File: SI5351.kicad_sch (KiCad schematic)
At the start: 21 parts, among them U10 SI5351B-B-GM1, Y1 25MHz

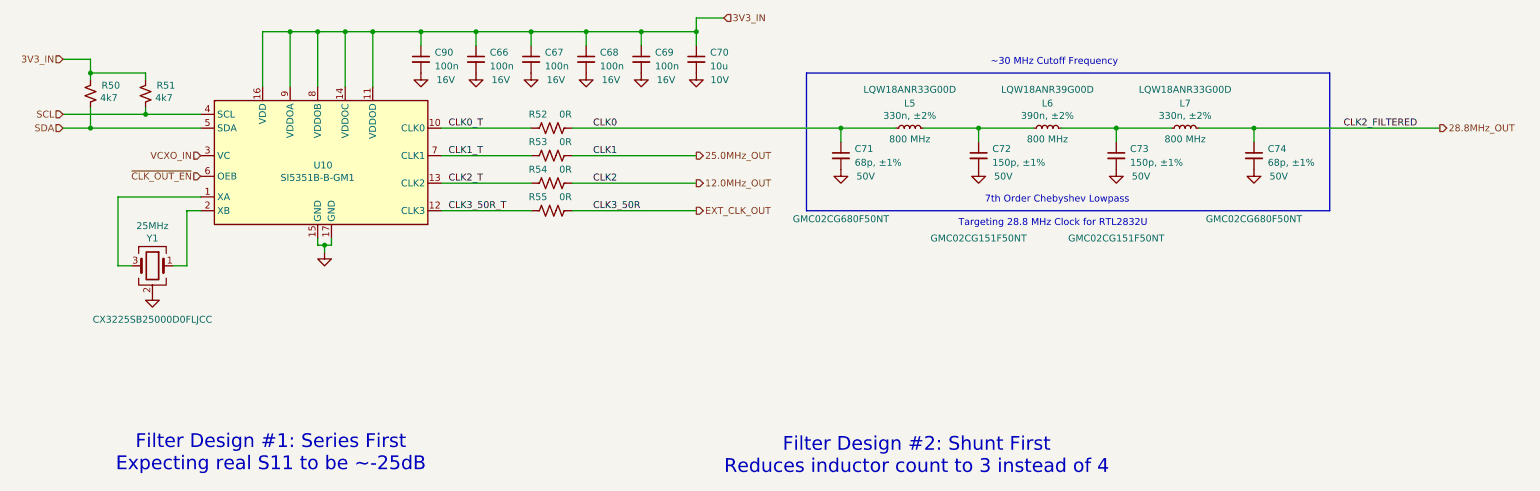
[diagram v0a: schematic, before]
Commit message: PCB and schematic progress
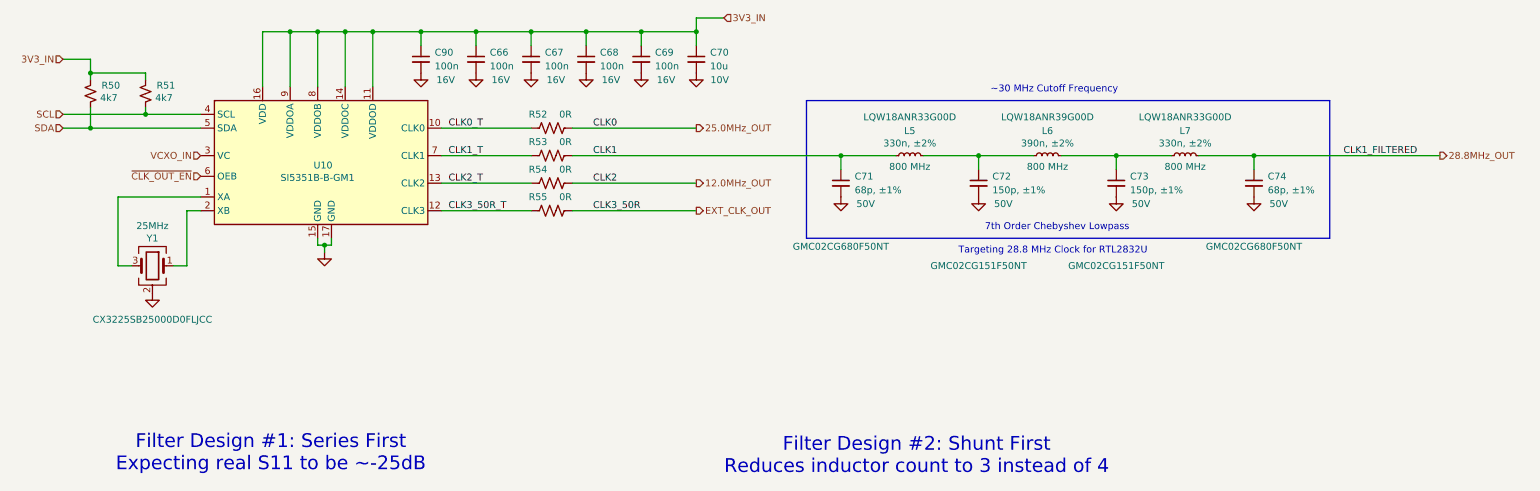
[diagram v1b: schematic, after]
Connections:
- net 25.0MHz_OUT: now also R52.2; no longer R53.2
- net CLK0 renamed CLK1
- net CLK1: now also R53.2; no longer R52.2
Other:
- moved on the sheet: C71, C72, C73, C74, L5, L6, L7
